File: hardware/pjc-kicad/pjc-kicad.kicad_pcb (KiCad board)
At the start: 2 copper layers, 113 x 106.7 mm, 88 parts, among them CON1 USB-MINI-B, CON10 CONN_2, CON2 CONN_3, CON3 CONN_2, CON4 M023.5MM, CON5 4PIN_FAN_CONN, CON6 CONN_2, CON7 CONN_2, CON8 AVR-ISP-10, CON9 CONN_2, Q1 MOSFET_P, Q2 RSQ045N03, SW1 SWITCH_INV, U1 VOM618A-4T, U10 NUD3124, U2 MCP3301, U3 FT232RL, U4 BSP762T, U5 ATMEGA328-P, U6 SN74LVC1G07, U7 L78M05C, U8 NUD3124, U9 TMP36_SOIC, X1 20MHz

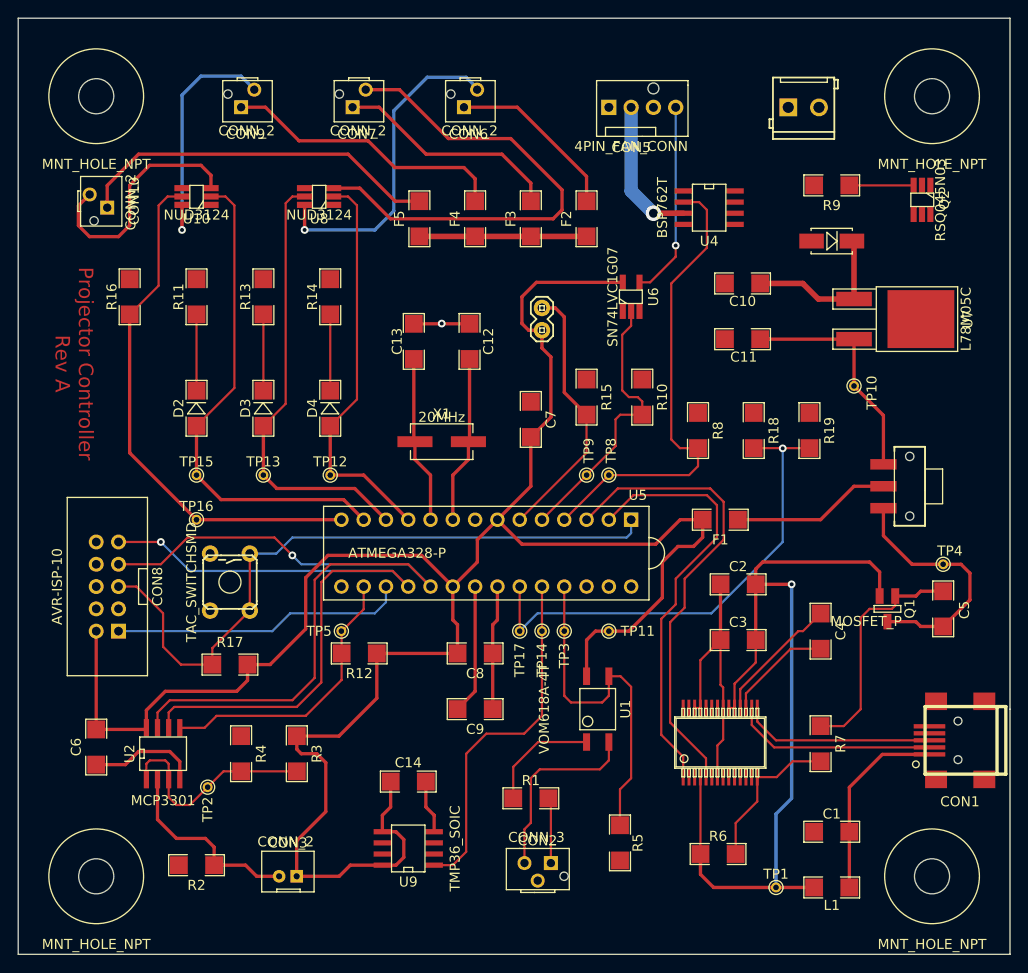
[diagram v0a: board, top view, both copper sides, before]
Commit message: Layout:  Almost there...
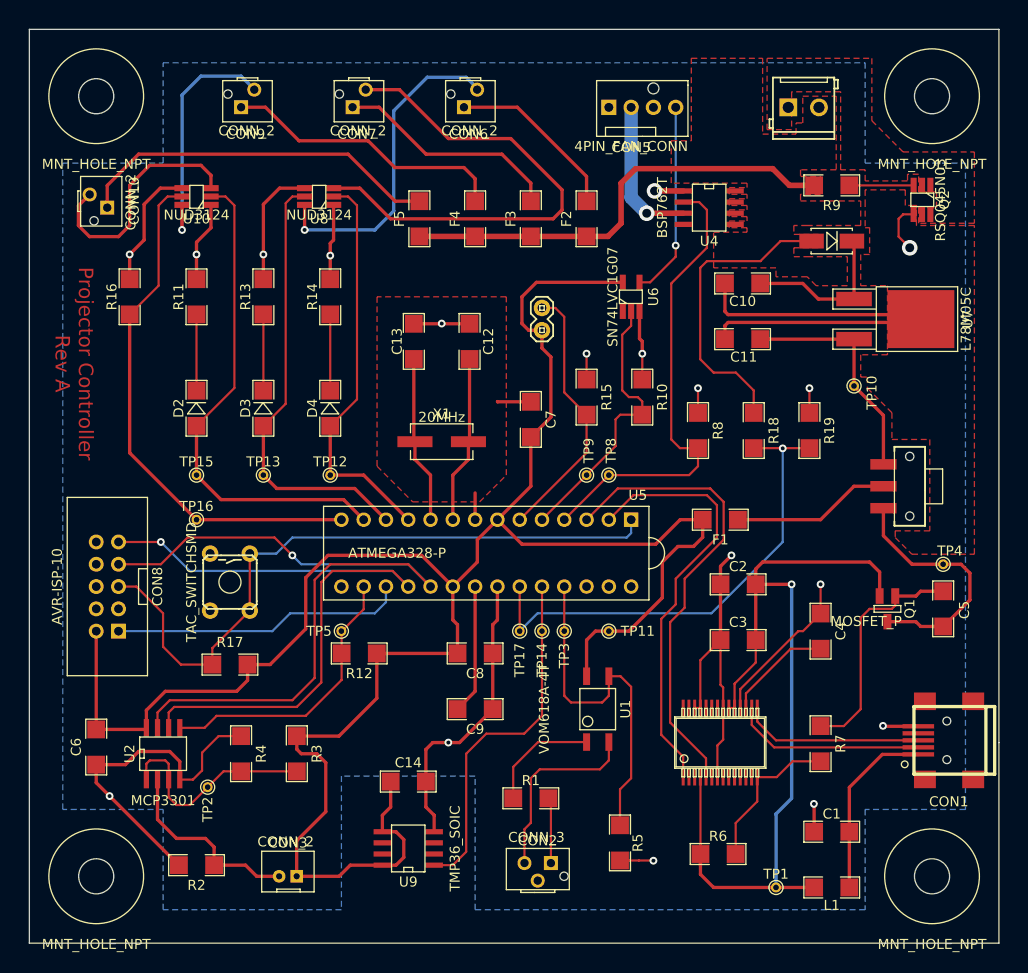
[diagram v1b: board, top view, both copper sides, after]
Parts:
- moved CON1 1.27 mm to (201.9, 129.3)
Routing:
- net GND: track 85.9 -> 271.5 mm, vias 1 -> 18
- net +12V: track 19.1 -> 86.1 mm
- net N-0000044: track 22.1 -> 20.8 mm
- net N-0000027: track 22.1 -> 20.8 mm
- net N-0000026: track 23.2 -> 22.0 mm
- added copper zone on F.Cu, net +12V
- added copper zone on B.Cu, net GND
- added copper zone on F.Cu, net GND
- added copper zone on F.Cu, net N-0000064
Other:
- board size 113 x 106.7 mm -> 110.5 x 104.1 mm
